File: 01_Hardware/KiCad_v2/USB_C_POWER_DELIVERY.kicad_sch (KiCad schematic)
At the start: 36 parts, among them Q200 SI7615DN-T1-GE3, Q201 SI7615DN-T1-GE3, Q202 DMP6050SSD-13, Q203 IRLML2402TRPBF, U200 CYPD3177-24LQ

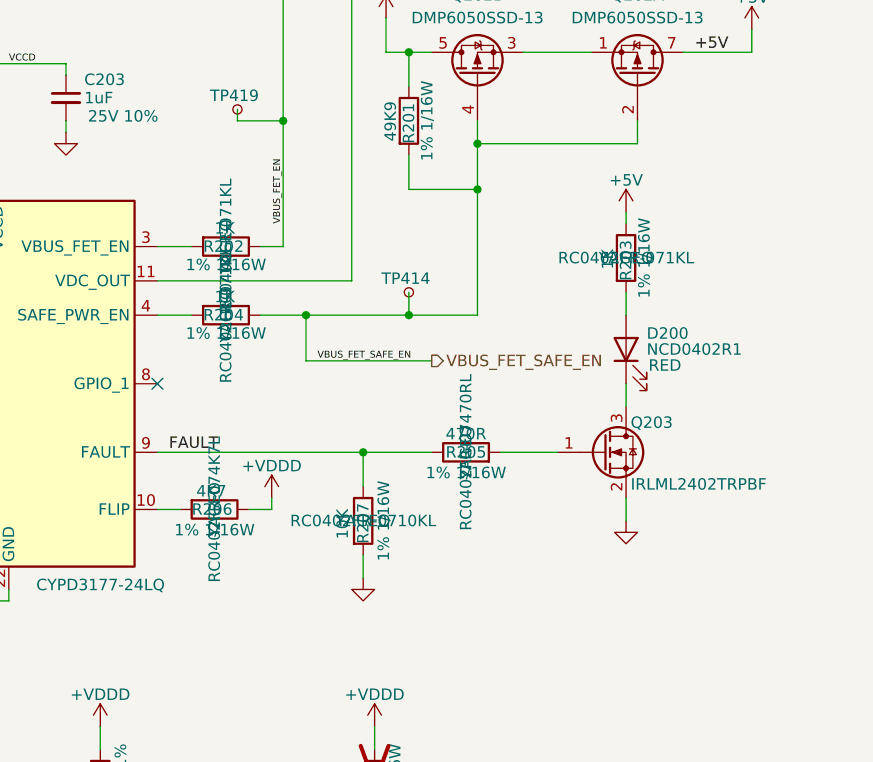
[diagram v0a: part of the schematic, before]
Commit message: USB-C and Serial PCB routing done
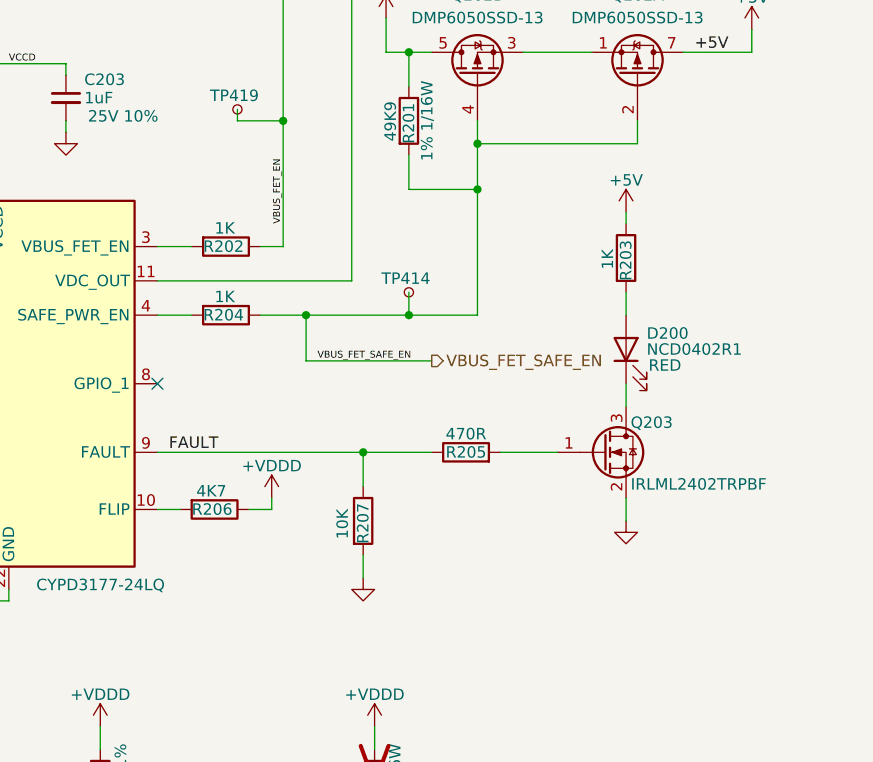
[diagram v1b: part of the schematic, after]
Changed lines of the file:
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@@
 					(size 1.27 1.27)
 				)
+				(hide yes)
 			)
 		)
@@
 					(size 1.27 1.27)
 				)
+				(hide yes)
 			)
 		)
@@
 					(size 1.27 1.27)
 				)
+				(hide yes)
 			)
 		)
@@
 					(size 1.27 1.27)
 				)
+				(hide yes)
 			)
 		)
@@
 					(size 1.27 1.27)
 				)
+				(hide yes)
 			)
 		)
@@
 					(size 1.27 1.27)
 				)
+				(hide yes)
 			)
 		)
@@
 					(size 1.27 1.27)
 				)
+				(hide yes)
 			)
 		)
@@
 					(size 1.27 1.27)
 				)
+				(hide yes)
 			)
 		)
@@
 					(size 1.27 1.27)
 				)
+				(hide yes)
 			)
 		)
@@
 					(size 1.27 1.27)
 				)
+				(hide yes)
 			)
 		)
@@
 					(size 1.27 1.27)
 				)
+				(hide yes)
 			)
 		)
@@
 					(size 1.27 1.27)
 				)
+				(hide yes)
 			)
 		)
@@
 					(size 1.27 1.27)
 				)
+				(hide yes)
 			)
 		)
@@
 					(size 1.27 1.27)
 				)
+				(hide yes)
 			)
 		)
@@
 					(size 1.27 1.27)
 				)
+				(hide yes)
 			)
 		)
@@
 					(size 1.27 1.27)
 				)
+				(hide yes)
 			)
 		)
@@
 					(size 1.27 1.27)
 				)
+				(hide yes)
 			)
 		)
@@
 					(size 1.27 1.27)
 				)
+				(hide yes)
 			)
 		)
@@
 					(size 1.27 1.27)
 				)
+				(hide yes)
 			)
 		)
@@
 					(size 1.27 1.27)
 				)
+				(hide yes)
 			)
 		)
@@
 					(size 1.27 1.27)
 				)
+				(hide yes)
 			)
 		)
@@
 					(size 1.27 1.27)
 				)
+				(hide yes)
 			)
 		)
@@
 					(size 1.27 1.27)
 				)
+				(hide yes)
 			)
 		)
@@
 					(size 1.27 1.27)
 				)
+				(hide yes)
 			)
 		)
@@
 					(size 1.27 1.27)
 				)
+				(hide yes)
 			)
 		)
@@
 					(size 1.27 1.27)
 				)
+				(hide yes)
 			)
 		)
@@
 					(size 1.27 1.27)
 				)
+				(hide yes)
 			)
 		)
@@
 					(size 1.27 1.27)
 				)
+				(hide yes)
 			)
 		)
@@
 					(size 1.27 1.27)
 				)
+				(hide yes)
 			)
 		)
@@
 					(size 1.27 1.27)
 				)
+				(hide yes)
 			)
 		)

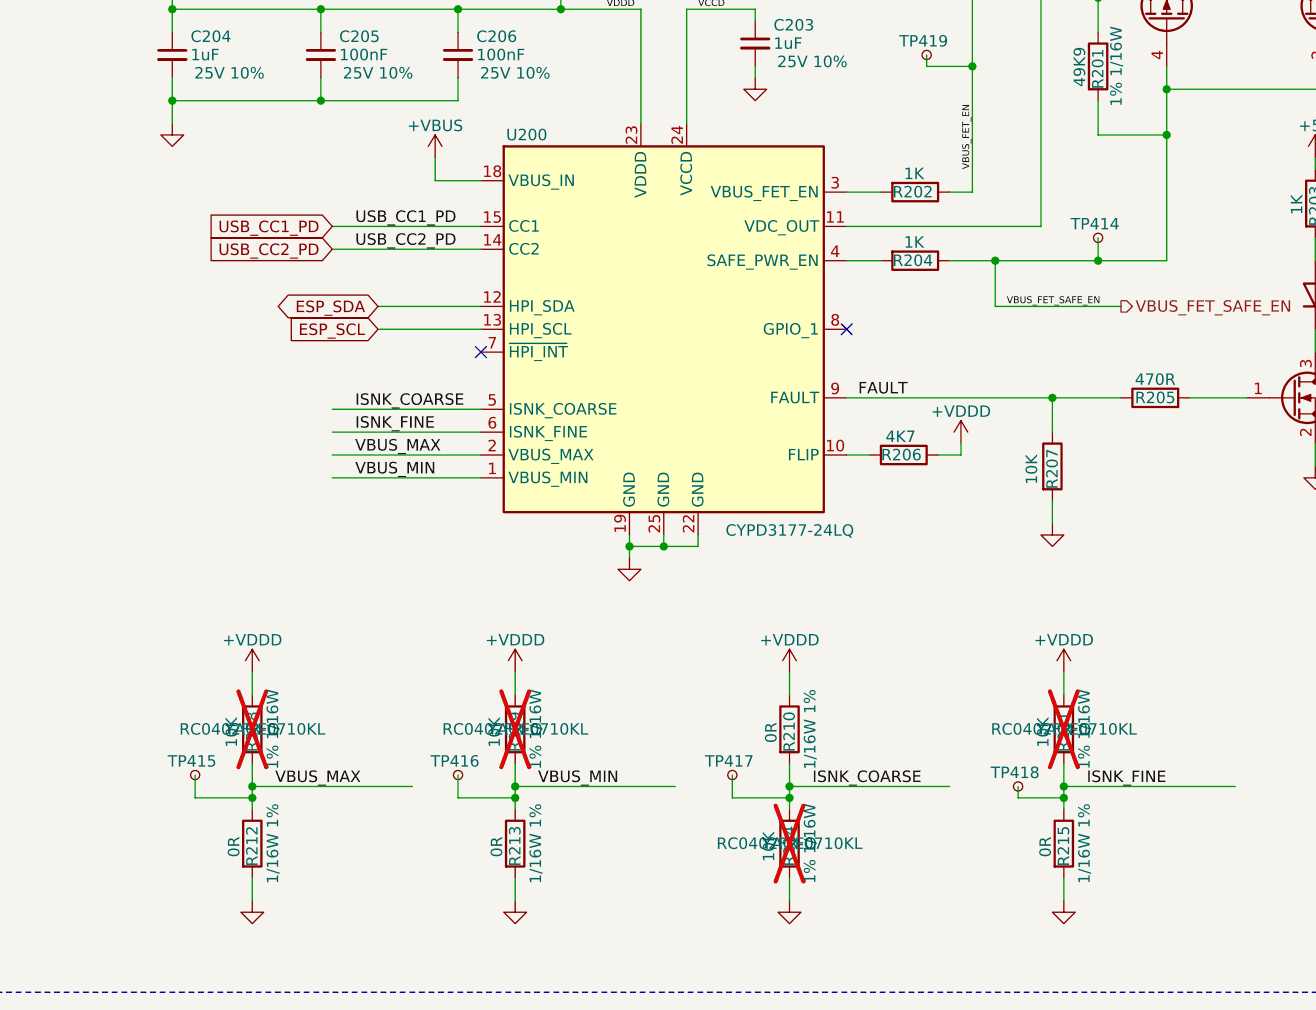
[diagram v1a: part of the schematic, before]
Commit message: PCB desing in progresssss
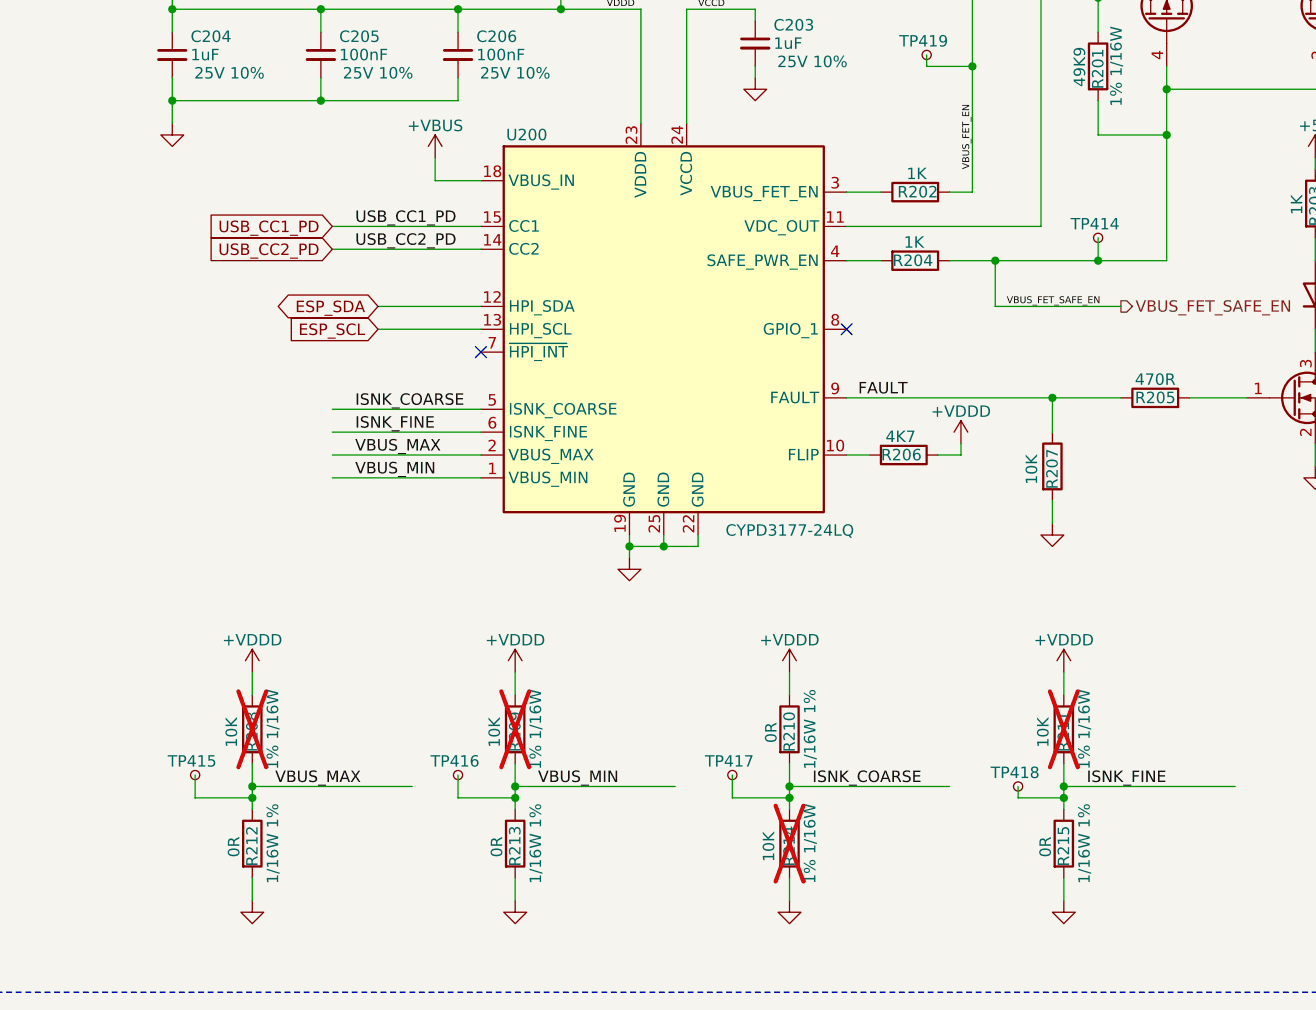
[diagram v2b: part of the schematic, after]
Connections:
- net VBUS_FET_EN: now also R202.2; no longer R202.1
- net at U200.3 (VBUS_FET_EN): now also R202.1; no longer R202.2
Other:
- moved on the sheet: R202
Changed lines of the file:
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@@
 					(size 1.27 1.27)
 				)
+				(hide yes)
 			)
 		)
@@
 					(size 1.27 1.27)
 				)
+				(hide yes)
 			)
 		)
@@
 					(size 1.27 1.27)
 				)
+				(hide yes)
 			)
 		)
@@
 					(size 1.27 1.27)
 				)
+				(hide yes)
 			)
 		)
@@
 					(size 1.27 1.27)
 				)
+				(hide yes)
 			)
 		)
@@
 					(size 1.27 1.27)
 				)
+				(hide yes)
 			)
 		)
@@
 					(size 1.27 1.27)
 				)
+				(hide yes)
 			)
 		)
@@
 					(size 1.27 1.27)
 				)
+				(hide yes)
 			)
 		)
@@
 					(size 1.27 1.27)
 				)
+				(hide yes)
 			)
 		)
@@
 					(size 1.27 1.27)
 				)
+				(hide yes)
 			)
 		)
@@
 					(size 1.27 1.27)
 				)
+				(hide yes)
 			)
 		)
@@
 					(size 1.27 1.27)
 				)
+				(hide yes)
 			)
 		)
@@
 	(symbol
 		(lib_id "Device:R")
-		(at 163.83 74.93 270)
+		(at 163.83 74.93 90)
+		(mirror x)
 		(unit 1)
 		(exclude_from_sim no)
@@
 		(dnp no)
 		(property "Reference" "R202"
-			(at 161.29 74.93 90)
+			(at 166.37 74.93 90)
 			(effects
 				(font
@@
 		)
 		(property "Value" "1K"
-			(at 162.56 72.898 90)
+			(at 165.1 72.898 90)
 			(effects
 				(font
@@
 					(size 1.27 1.27)
 				)
+				(hide yes)
 			)
 		)
@@
 					(size 1.27 1.27)
 				)
+				(hide yes)
 			)
 		)
@@
 					(size 1.27 1.27)
 				)
+				(hide yes)
 			)
 		)
@@
 					(size 1.27 1.27)
 				)
+				(hide yes)
 			)
 		)
